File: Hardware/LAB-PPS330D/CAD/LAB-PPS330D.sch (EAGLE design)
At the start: 8 parts, among them J1 100mil, J2 100mil, U1 SN74LVC1G139, U2 ADP1196, U3 ADP1196, U4 ADP1196, U5 ADP1196, U6 SN74LVC3G04DCURBGA

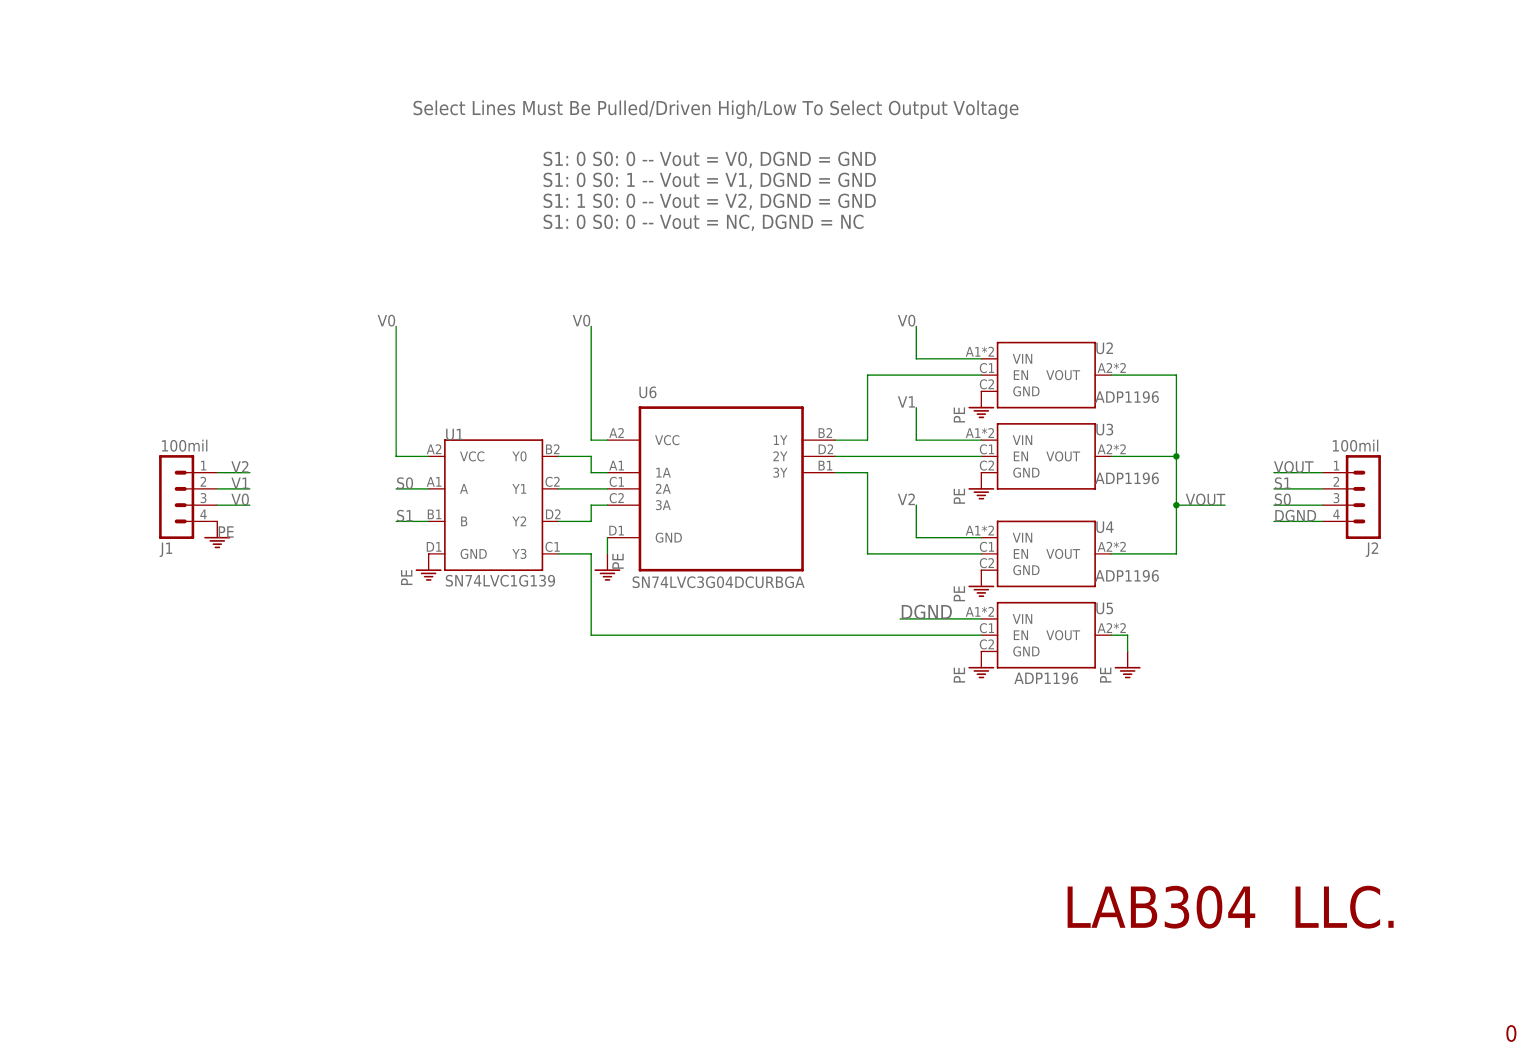
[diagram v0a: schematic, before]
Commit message: 1) This is the final Rev1 version going off to MFG
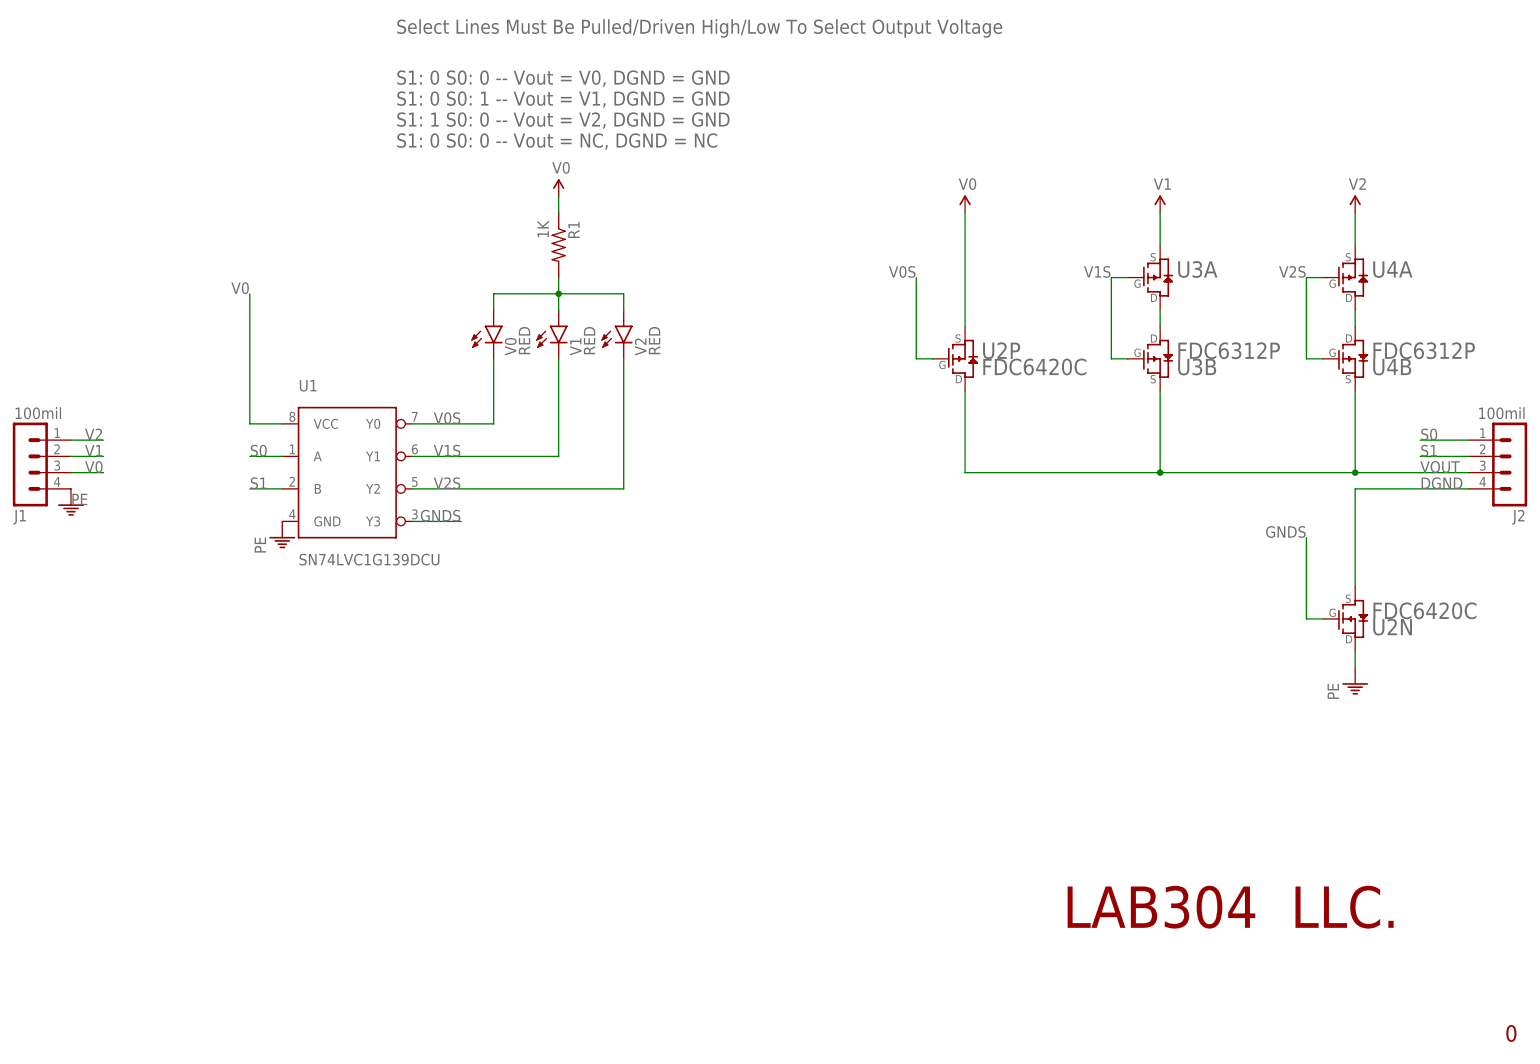
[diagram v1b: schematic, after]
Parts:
- removed U5: ADP1196, My Library-adm:ADP1196
- removed U6: SN74LVC3G04DCURBGA, My Library-adm:SN74LVC3G04DCURBGA
- added R1: 1K, SparkFun-Resistors:1KOHM-1/10W-1%(0603)
- added V0, V1, V2: RED, SparkFun-LED:LED-RED0603
- U1: value SN74LVC1G139 -> SN74LVC1G139DCU; device My Library-adm:SN74LVC1G139 -> LAB-PPS330D:SN74LVC1G139DCU
- U2: value ADP1196 -> FDC6420C; device My Library-adm:ADP1196 -> LAB-PPS330D:FDC6420C
- U3, U4: value ADP1196 -> FDC6312P; device My Library-adm:ADP1196 -> LAB-PPS330D:FDC6312P
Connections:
- removed net N$3: U4.EN, U6.3Y
- removed net N$4: U1.Y0, U6.1A
- removed net N$6: U1.Y2, U6.3A
- removed net N$7: U1.Y3, U5.EN
- new net GNDS: U1.Y3, U2N.G
- new net V0S: U1.Y0, U2P.G, V0.C
- new net V1S: U1.Y1, U3A.G, U3B.G, V1.C
- new net V2S: U1.Y2, U4A.G, U4B.G, V2.C
- net DGND: now also U2N.S; no longer U5.VIN
- net N$1: now also U3A.D, U3B.D; no longer U2.EN, U6.1Y
- net N$2: now also U4A.D, U4B.D; no longer U3.EN, U6.2Y
- net N$5: now also R1.2, V0.A, V1.A, V2.A; no longer U1.Y1, U6.2A
- net PE: now also U2N.D; no longer U2.GND, U3.GND, U4.GND, U5.GND, U5.VOUT, U6.GND
- net S0: now also J2.1; no longer J2.3
- net V0: now also R1.1, U2P.S; no longer U2.VIN, U6.VCC
- net V1: now also U3A.S; no longer U3.VIN
- net V2: now also U4A.S; no longer U4.VIN
- net VOUT: now also J2.3, U2P.D, U3B.S, U4B.S; no longer J2.1, U2.VOUT, U3.VOUT, U4.VOUT
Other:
- note removed: "SN74LVC1G139"
- note removed: "U1"
- moved on the sheet: J1, J2
